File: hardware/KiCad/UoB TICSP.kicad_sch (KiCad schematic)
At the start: 30 parts, among them J1 Wago 233-503, J2 Conn_01x01_Pin, J3 Conn_01x01_Pin, J4 Conn_01x01_Pin, J5 Conn_01x01_Pin, J6 SMA, J7 SMA, U6 LM317_SOT-223, U7 LM337_SOT223

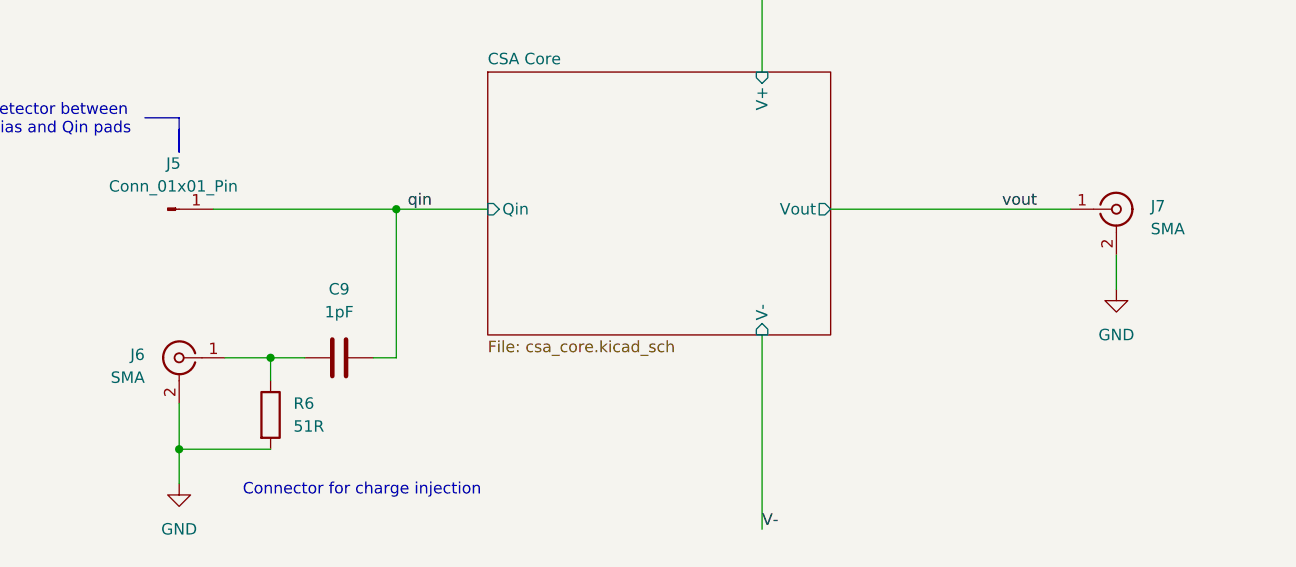
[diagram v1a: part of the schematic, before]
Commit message: Printed PDF schemaics. Saved schematic and PCB as KiCAD 9
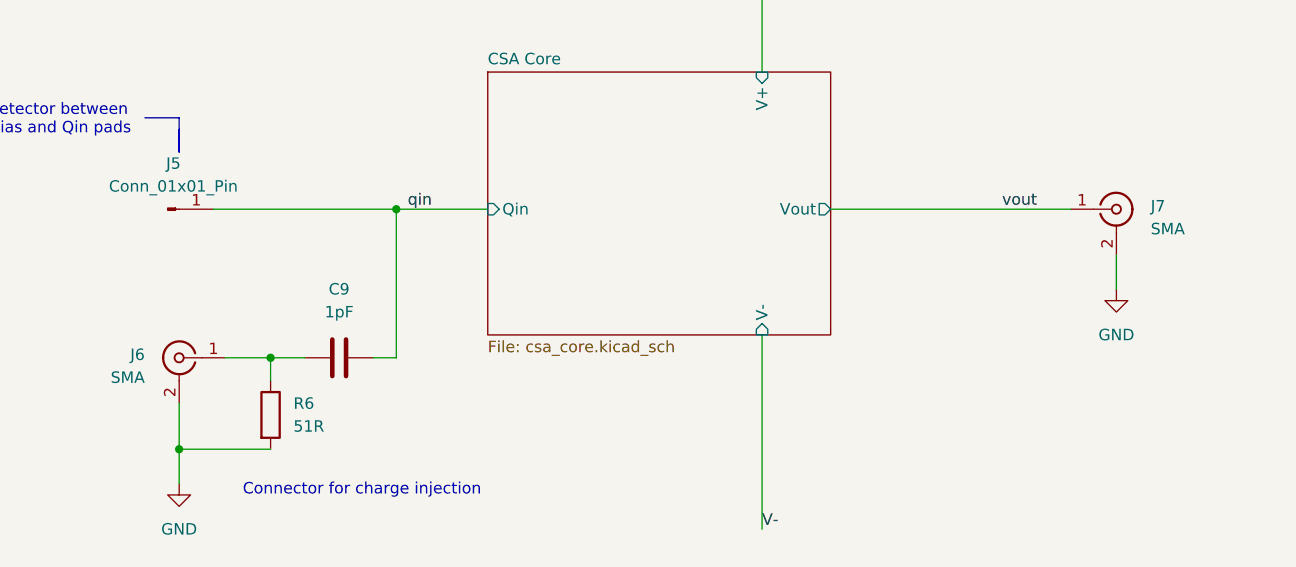
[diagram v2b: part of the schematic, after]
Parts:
- C9: value 1pF -> 1pF
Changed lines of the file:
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@@
 (kicad_sch
-	(version 20231120)
+	(version 20250114)
 	(generator "eeschema")
-	(generator_version "8.0")
+	(generator_version "9.0")
 	(paper "A4")
+	(text "CSA + Shaping Amplifier\n"
+		(exclude_from_sim no)
+		(at 190.5 190.5 0)
+		(effects
+			(font
+				(size 1.27 1.27)
+			)
+			(justify left bottom)
+		)
+	)
+	(text "Ian Bickerton CEng"
+		(exclude_from_sim no)
+		(at 226.06 196.85 0)
+		(effects
+			(font
+				(size 1.27 1.27)
+			)
+			(justify left bottom)
+		)
+	)
+	(text "Connector for charge injection"
+		(exclude_from_sim no)
+		(at 158.75 148.082 0)
+		(effects
+			(font
+				(size 1.27 1.27)
+			)
+		)
+	)
+	(text "Detector bias up to 2.5kV"
+		(exclude_from_sim no)
+		(at 89.408 157.988 0)
+		(effects
+			(font
+				(size 1.27 1.27)
+			)
+		)
+	)
+	(text "Charge sensitive amplifier with shaping amplifiers\napproximately 5mV / fC\n\nPower supply from Ian Bickerstaff \n"
+		(exclude_from_sim no)
+		(at 180.34 180.34 0)
+		(effects
+			(font
+				(size 2 2)
+			)
+			(justify left bottom)
+		)
+	)
+	(text "1"
+		(exclude_from_sim no)
+		(at 270.51 194.31 0)
+		(effects
+			(font
+				(size 1.27 1.27)
+			)
+			(justify left bottom)
+		)
+	)
+	(text "Connect detector between\ndetector_bias and Qin pads"
+		(exclude_from_sim no)
+		(at 121.158 106.934 0)
+		(effects
+			(font
+				(size 1.27 1.27)
+			)
+		)
+	)
+	(text "April 2023"
+		(exclude_from_sim no)
+		(at 209.55 194.31 0)
+		(effects
+			(font
+				(size 1.27 1.27)
+			)
+			(justify left bottom)
+		)
+	)
 	(junction
 		(at 74.93 139.7)
@@
 		)
 	)
-	(text "CSA + Shaping Amplifier\n"
-		(exclude_from_sim no)
-		(at 190.5 190.5 0)
-		(effects
-			(font
-				(size 1.27 1.27)
-			)
-			(justify left bottom)
-		)
-	)
-	(text "Ian Bickerton CEng"
-		(exclude_from_sim no)
-		(at 226.06 196.85 0)
-		(effects
-			(font
-				(size 1.27 1.27)
-			)
-			(justify left bottom)
-		)
-	)
-	(text "Connector for charge injection"
-		(exclude_from_sim no)
-		(at 158.75 148.082 0)
-		(effects
-			(font
-				(size 1.27 1.27)
-			)
-		)
-	)
-	(text "Detector bias up to 2.5kV"
-		(exclude_from_sim no)
-		(at 89.408 157.988 0)
-		(effects
-			(font
-				(size 1.27 1.27)
-			)
-		)
-	)
-	(text "Charge sensitive amplifier with shaping amplifiers\napproximately 5mV / fC\n\nPower supply from Ian Bickerstaff \n"
-		(exclude_from_sim no)
-		(at 180.34 180.34 0)
-		(effects
-			(font
-				(size 2 2)
-			)
-			(justify left bottom)
-		)
-	)
-	(text "1"
-		(exclude_from_sim no)
-		(at 270.51 194.31 0)
-		(effects
-			(font
-				(size 1.27 1.27)
-			)
-			(justify left bottom)
-		)
-	)
-	(text "Connect detector between\ndetector_bias and Qin pads"
-		(exclude_from_sim no)
-		(at 121.158 106.934 0)
-		(effects
-			(font
-				(size 1.27 1.27)
-			)
-		)
-	)
-	(text "April 2023"
-		(exclude_from_sim no)
-		(at 209.55 194.31 0)
-		(effects
-			(font
-				(size 1.27 1.27)
-			)
-			(justify left bottom)
-		)
-	)
 	(label "+12V"
 		(at 33.02 53.34 0)
-		(fields_autoplaced yes)
 		(effects
 			(font
@@
 	(label "+10V"
 		(at 115.57 27.94 0)
-		(fields_autoplaced yes)
 		(effects
 			(font
@@
 	(label "-9V"
 		(at 33.02 58.42 0)
-		(fields_autoplaced yes)
 		(effects
 			(font
@@
 	(label "V-"
 		(at 116.84 85.09 0)
-		(fields_autoplaced yes)
 		(effects
 			(font
@@
 	(label "bias_in"
 		(at 78.74 152.4 0)
-		(fields_autoplaced yes)
 		(effects
 			(font
@@
 	(label "bias_filt"
 		(at 74.93 140.97 0)
-		(fields_autoplaced yes)
 		(effects
 			(font
@@
 	(label "detector_bias"
 		(at 80.01 116.84 0)
-		(fields_autoplaced yes)
 		(effects
 			(font
@@
 	(label "V-"
 		(at 203.2 152.4 0)
-		(fields_autoplaced yes)
 		(effects
 			(font
@@
 	(label "vout"
 		(at 229.87 116.84 0)
-		(fields_autoplaced yes)
 		(effects
 			(font
@@
 	(label "+10V"
 		(at 203.2 85.09 0)
-		(fields_autoplaced yes)
 		(effects
 			(font
@@
 	(label "GND"
 		(at 34.29 55.88 0)
-		(fields_autoplaced yes)
 		(effects
 			(font
@@
 	(label "qin"
 		(at 163.83 116.84 0)
-		(fields_autoplaced yes)
 		(effects
 			(font
@@
 			)
 		)
-		(property "Value" "1pF	"
+		(property "Value" "1pF"
 			(at 156.21 128.27 90)
 			(effects
@@
 		(at 172.72 101.6)
 		(size 38.1 29.21)
+		(exclude_from_sim no)
+		(in_bom yes)
+		(on_board yes)
+		(dnp no)
 		(fields_autoplaced yes)
 		(stroke
@@
 		)
 	)
+	(embedded_fonts no)
 )
